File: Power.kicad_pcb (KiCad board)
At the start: 4 copper layers, 138.7 x 119.4 mm, 50 parts, among them J1 OUT-, J2 OUT+, J3 IN+, J4 IN-, J5 Conn_02x05_Odd_Even, U1 TMR_1-0511

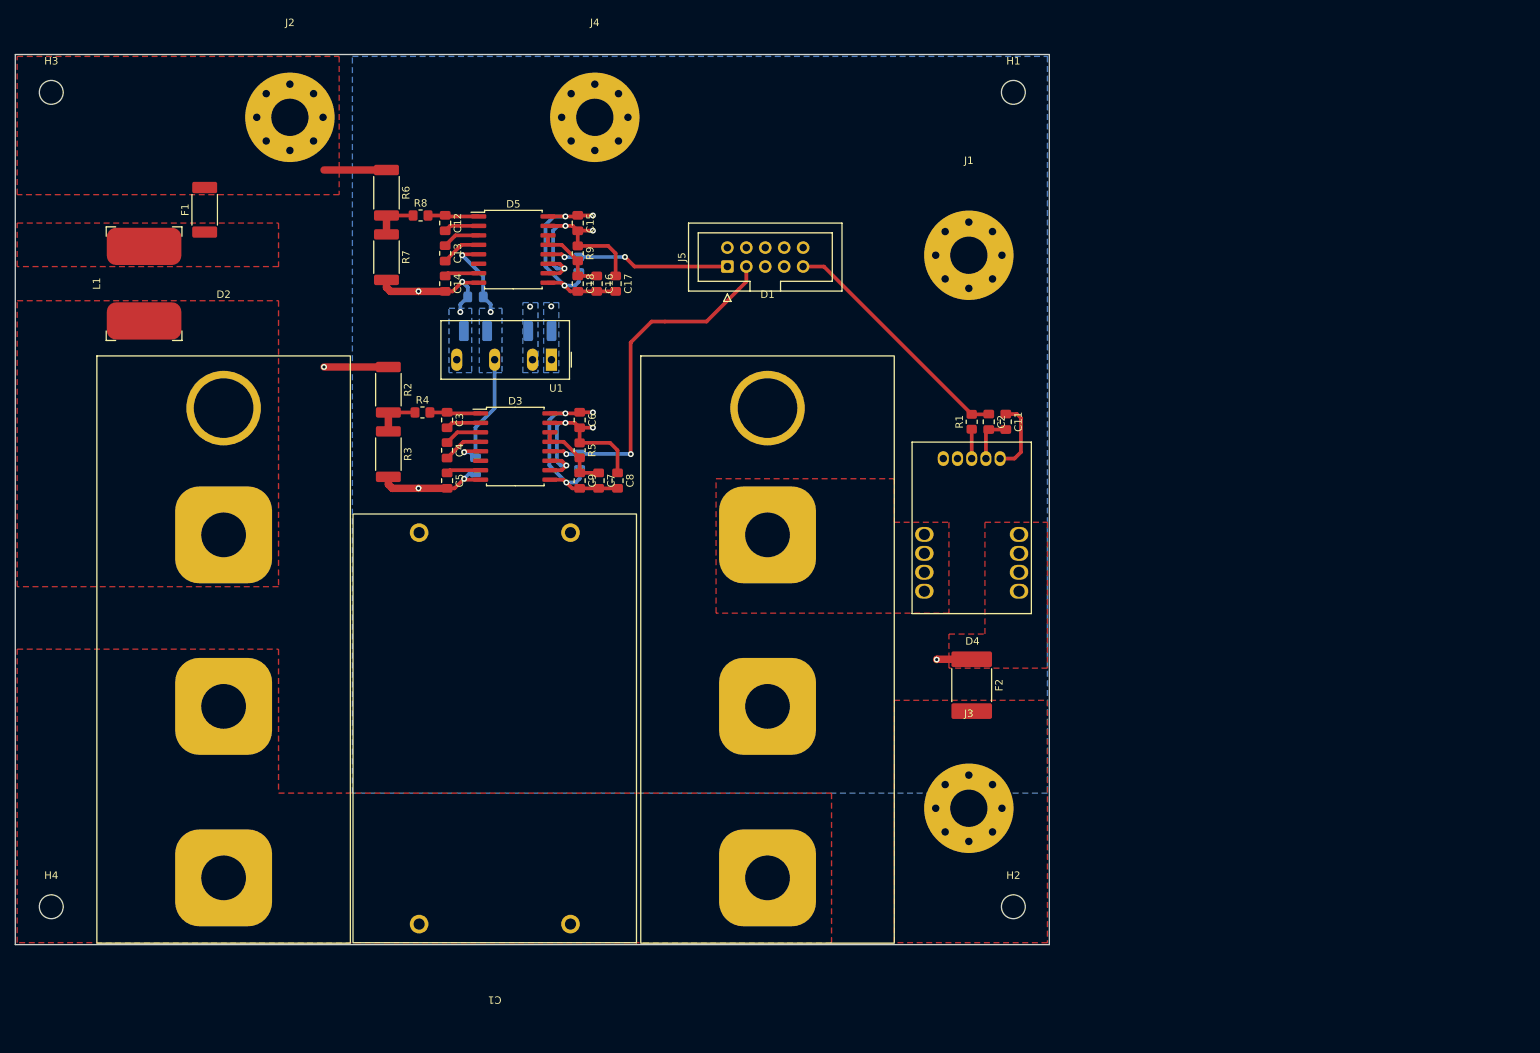
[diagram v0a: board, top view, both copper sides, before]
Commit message: VER2.0
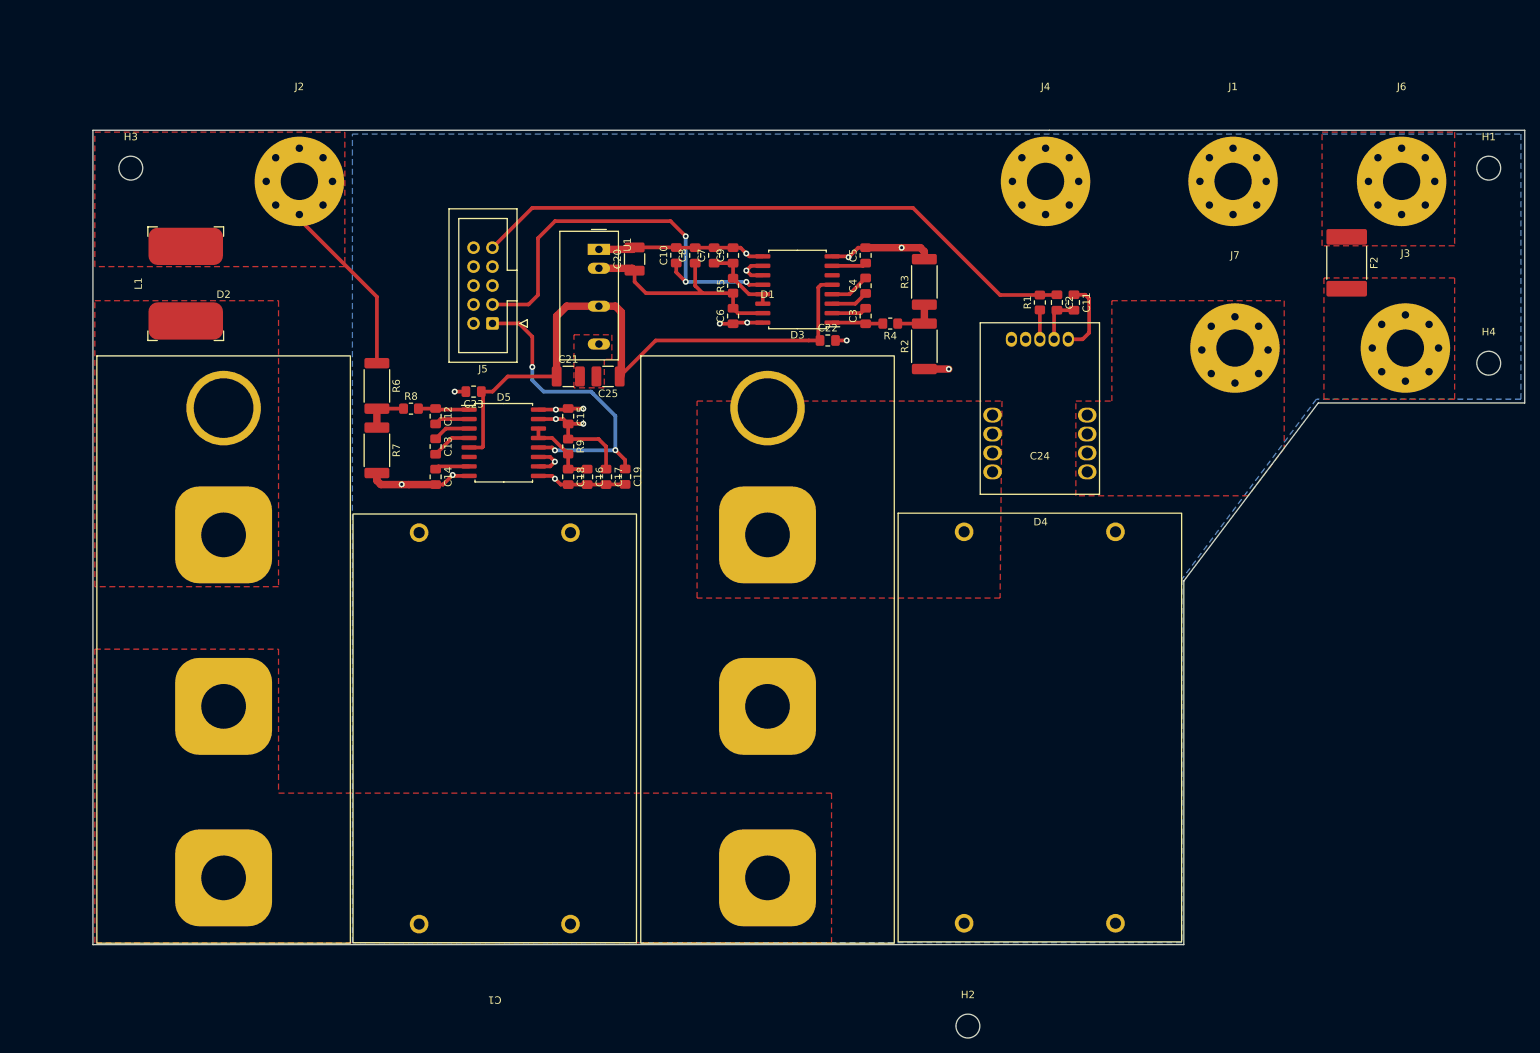
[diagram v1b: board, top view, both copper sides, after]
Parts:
- removed F1: Fuse, Fuse:Fuse_2512_6332Metric_Pad1.52x3.35mm_HandSolder
- added C24: 100u, Capacitor_4pin:C4AE, F.Cu at (161.8, 82.1)
- added C25: C_Small, Capacitor_SMD:C_1210_3225Metric_Pad1.33x2.70mm_HandSolder, F.Cu at (102.6, 63.8)
- added J6: L_IN, Connector Power:M5, F.Cu at (209.0, 37.6)
- added J7: L_OUT, Connector Power:M5, F.Cu at (186.7, 60.2)
- C10, C19, C20, C21, C22, C23: moved to F.Cu
- moved H4 206.1 mm to (220.7, 62.0)
- moved J3 85.1 mm to (209.6, 59.9)
- moved F2 75.7 mm to (201.7, 48.5)
- moved R3 75.5 mm to (145.0, 51.1), turned to 90 degrees
- moved R2 72.1 mm to (145.0, 59.7), turned to 90 degrees
- moved H1 64.6 mm to (220.7, 35.8)
- moved R4 63.9 mm to (140.5, 56.7), turned to 180 degrees
- moved C5 63.7 mm to (137.2, 47.5), turned to 90 degrees
- moved J4 61.1 mm to (161.3, 37.6)
- moved C4 60.3 mm to (137.2, 51.6), turned to 90 degrees
- moved C3 57.8 mm to (137.2, 55.6), turned to 90 degrees
- moved C22 50.1 mm to (132.1, 58.9), turned to 0 degrees
- moved D3 43.3 mm to (128.0, 52.1), turned to 180 degrees
- moved J1 36.8 mm to (186.4, 37.6)
- moved C9 36.5 mm to (119.4, 47.5), turned to 90 degrees
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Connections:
- F2 pad 1: /input current -> /IN+
- L1 pad 2: Net-(L1-Pad2) -> /OUT+
- R2 pad 1: /input current -> /IN+
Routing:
- net /input current: track 125.5 -> 0.00 mm, vias 2 -> 0
- net +5VP: track 29.8 -> 85.1 mm, vias 3 -> 0
- net /Current_measure: track 33.1 -> 82.8 mm
- net /Output_Voltage: track 24.6 -> 43.2 mm, vias 2 -> 3
- net /OUT+: track 8.38 -> 23.6 mm
- net GND: track 68.0 -> 53.0 mm, vias 7 -> 6
- net /IN+: track 0.00 -> 11.1 mm, vias 0 -> 1
- net /Input_Voltage: track 46.9 -> 55.5 mm, vias 2 -> 3
- net GNDPWR: track 35.1 -> 31.4 mm, vias 5 -> 6
- net +5V: track 69.1 -> 67.7 mm, vias 7 -> 4
- added copper zone on In2.Cu, net +5V
- added copper zone on F.Cu, net /IN+
- added copper zone on In1.Cu, net /IN+
- added copper zone on In1.Cu, net GND
- added copper zone on F.Cu, net GNDPWR
- removed copper zone on B.Cu, net +5V
- removed copper zone on In1.Cu, net +5V
- removed copper zone on B.Cu, net +5VP
- removed copper zone on B.Cu, net GND
- removed copper zone on In2.Cu, net GND
- removed copper zone on F.Cu, net Net-(L1-Pad2)
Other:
- board size 138.7 x 119.4 mm -> 192 x 109.2 mm
